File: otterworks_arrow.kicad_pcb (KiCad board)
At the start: 4 copper layers, 60 x 121 mm, 308 parts, among them J1 PROG, SW1 SW_Push, U2 BHI160B, U3 STM32F030K6Tx

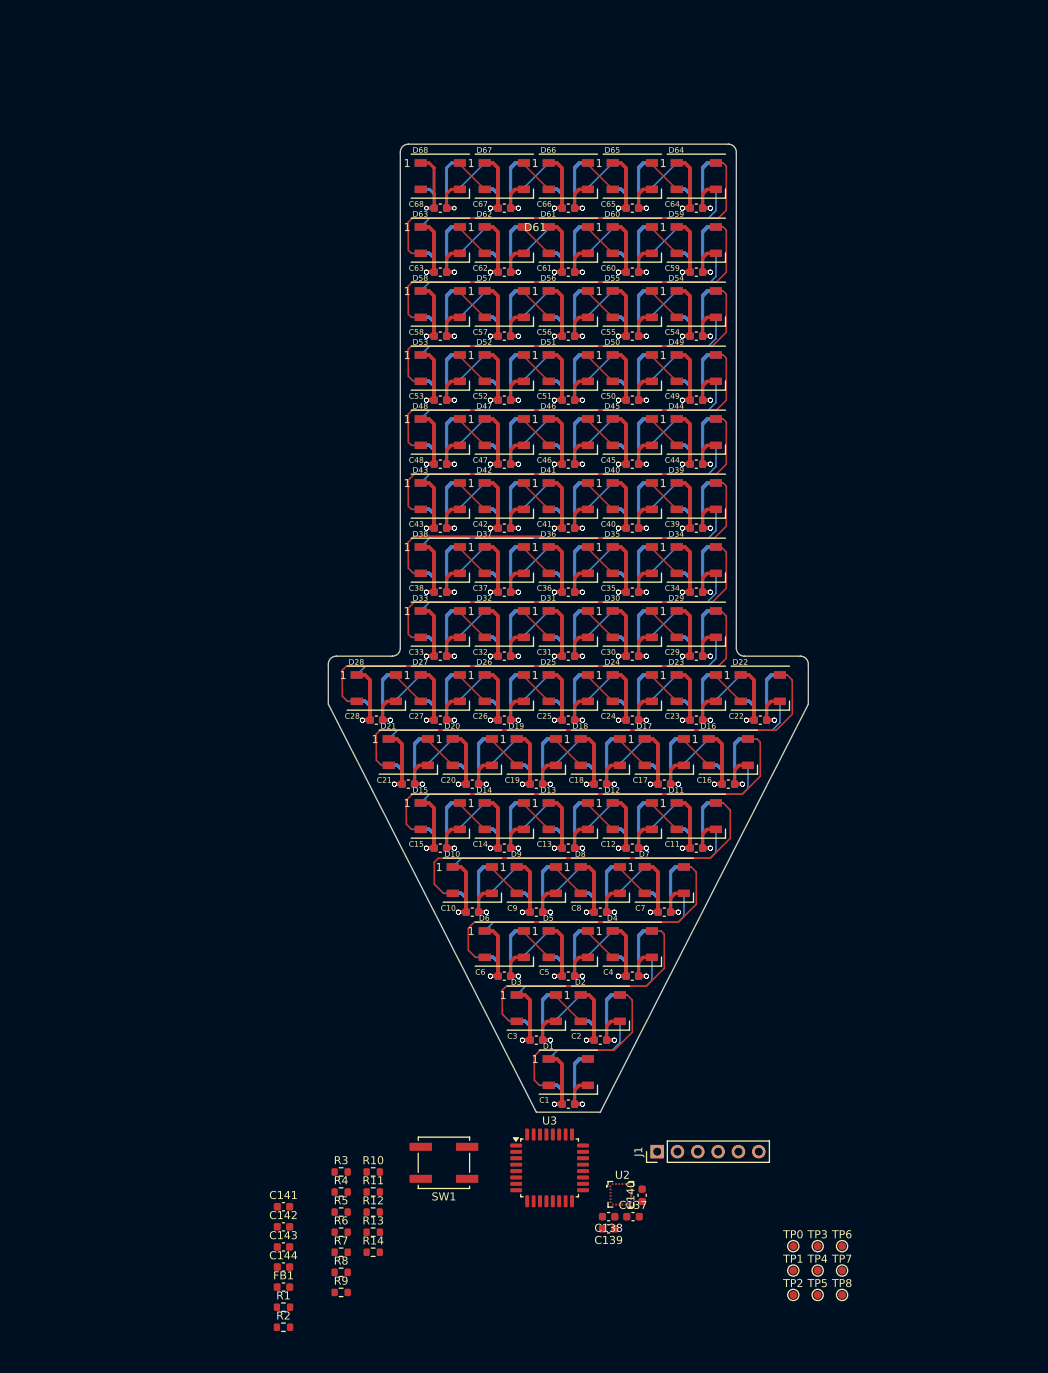
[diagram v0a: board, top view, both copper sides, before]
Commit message: wip
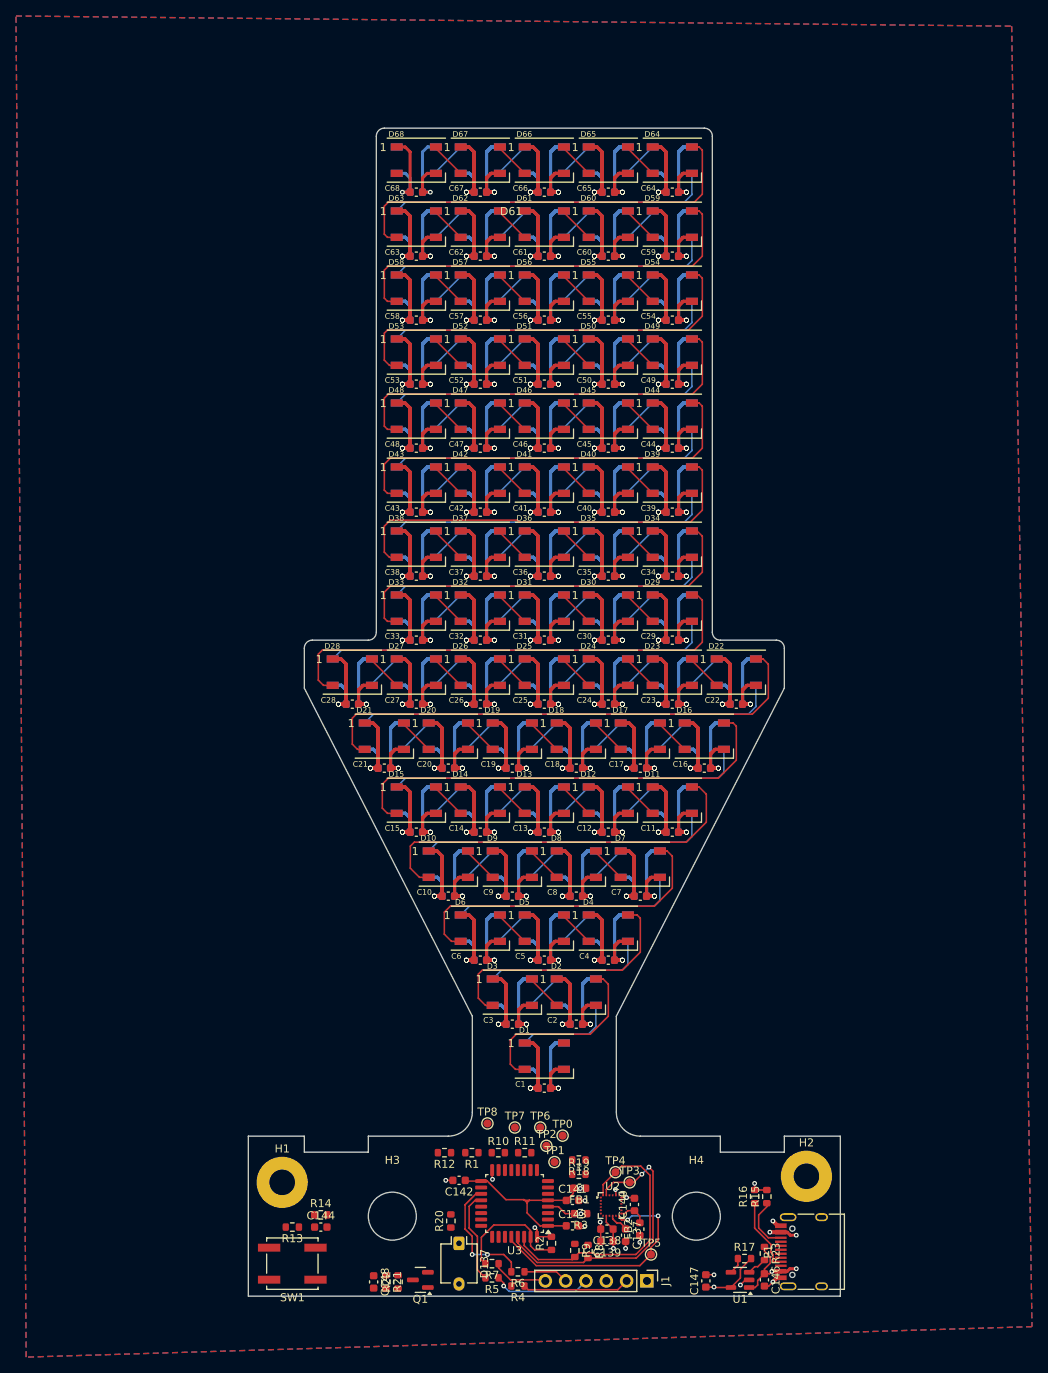
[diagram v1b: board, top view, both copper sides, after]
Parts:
- added C146: 100n, Capacitor_SMD:C_0603_1608Metric, F.Cu at (107.5, 163.0)
- added C147: 100n, Capacitor_SMD:C_0603_1608Metric, F.Cu at (100.2, 163.1)
- added C148: 100n, Capacitor_SMD:C_0603_1608Metric, F.Cu at (58.7, 163.2)
- added D137: BPW34, OptoDevice:Osram_DIL2_4.3x4.65mm_P5.08mm, F.Cu at (69.3, 158.4)
- added FB2: ferrite, Inductor_SMD:L_0603_1608Metric, F.Cu at (91.9, 156.6)
- added H1: MountingHole_Pad, MountingHole:MountingHole_3.2mm_M3_Pad, F.Cu at (47.2, 150.8)
- added H2: MountingHole_Pad, MountingHole:MountingHole_3.2mm_M3_Pad, F.Cu at (112.8, 150.0)
- added H3: MountingHole, MountingHole:MountingHole_6mm, F.Cu at (61.0, 155.0)
- added H4: MountingHole, MountingHole:MountingHole_6mm, F.Cu at (99.0, 155.0)
- added P1: USB_C_Plug_USB2.0, Connector_USB:USB_C_Receptacle_HRO_TYPE-C-31-M-12, F.Cu at (113.6, 159.4)
- added Q1: MMBT2484LT1G, Package_TO_SOT_SMD:SOT-23, F.Cu at (64.5, 163.0)
- added R15: 5.1k, Resistor_SMD:R_0603_1608Metric, F.Cu at (107.8, 152.6)
- added R16: 5.1k, Resistor_SMD:R_0603_1608Metric, F.Cu at (106.3, 152.6)
- added R17: 0, Resistor_SMD:R_0603_1608Metric, F.Cu at (105.0, 160.3)
- added R18: 33k, Resistor_SMD:R_0603_1608Metric, F.Cu at (84.3, 148.0)
- added R19: 10k, Resistor_SMD:R_0603_1608Metric, F.Cu at (84.3, 149.8)
- added R20: 10, Resistor_SMD:R_0603_1608Metric, F.Cu at (68.3, 155.6)
- added R21: 33k, Resistor_SMD:R_0603_1608Metric, F.Cu at (60.2, 163.2)
- added R22: 10k, Resistor_SMD:R_0603_1608Metric, F.Cu at (61.7, 163.2)
- added R23: 10k, Resistor_SMD:R_0603_1608Metric, F.Cu at (107.5, 159.7)
- added U1: ADP7142AUJZ-3.3, Package_TO_SOT_SMD:TSOT-23-5, F.Cu at (104.5, 163.0)
- moved TP8 49.2 mm to (72.9, 143.4)
- moved TP7 44.6 mm to (76.3, 143.9)
- moved TP6 40.5 mm to (79.5, 143.9)
- moved FB1 39.0 mm to (84.4, 151.5), turned to 180 degrees
- moved C143 36.2 mm to (83.5, 156.2)
- moved C141 36.1 mm to (83.5, 153.0)
- moved TP2 36.1 mm to (80.3, 146.2)
- moved R2 35.1 mm to (80.9, 158.4), turned to 90 degrees
- moved TP1 32.8 mm to (81.3, 148.2)
- moved TP0 32.0 mm to (82.3, 144.9)
- moved R8 31.0 mm to (85.5, 159.4), turned to -90 degrees
- moved R1 30.5 mm to (70.9, 147.1), turned to 180 degrees
- moved R3 30.4 mm to (84.5, 154.7), turned to 180 degrees
- moved R9 29.7 mm to (83.8, 159.3), turned to -90 degrees
- moved TP4 28.1 mm to (88.9, 149.5)
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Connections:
- net +3.3VA renamed Net-(U2-VDD)
- net Net-(U3-PA3) renamed /IN_SWITCH
- R9 pad 2: I2C1_SCL -> I2C1_SDA
- U3 pad 10: unconnected-(U3-PA4-Pad10) -> /IN_ADC_SUPPLY
- U3 pad 11: unconnected-(U3-PA5-Pad11) -> /IN_AMB_LIGHT
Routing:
- net I2C1_SCL: track 0.00 -> 36.5 mm, vias 0 -> 2
- net I2C1_SDA: track 0.00 -> 35.5 mm
- net I2C1_INT: track 0.00 -> 30.4 mm, vias 0 -> 2
- net Net-(U3-VDDA): track 0.00 -> 23.4 mm
- net GND: track 3076.2 -> 3097.1 mm, vias 269 -> 283
- net PROG_TX: track 0.00 -> 15.7 mm, vias 0 -> 2
- net PROG_BOOT0: track 0.00 -> 15.3 mm
- net +3.3V: track 0.00 -> 15.2 mm, vias 0 -> 5
- net +5V: track 2857.0 -> 2871.6 mm, vias 269 -> 273
- net Net-(J1-Pin_2): track 0.00 -> 13.4 mm
- net Net-(J1-Pin_4): track 0.00 -> 12.4 mm, vias 0 -> 1
- net PROG_RX: track 0.00 -> 11.6 mm
- net Net-(P1-CC): track 0.00 -> 9.22 mm
- net Net-(J1-Pin_6): track 0.00 -> 7.06 mm
- net Net-(P1-VCONN): track 0.00 -> 6.80 mm
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- added copper zone on In2.Cu, net +3.3V
- added copper zone on B.Cu, net GND
- added copper zone on F.Cu, net GND
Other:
- board size 60 x 121 mm -> 74 x 146 mm
